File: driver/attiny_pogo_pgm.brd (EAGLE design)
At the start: 26.9 x 17.3 mm, 9 parts, among them IC1 ATTiny85, J1 AVR_SPI_PRG_6NS, P5V TPTP10R

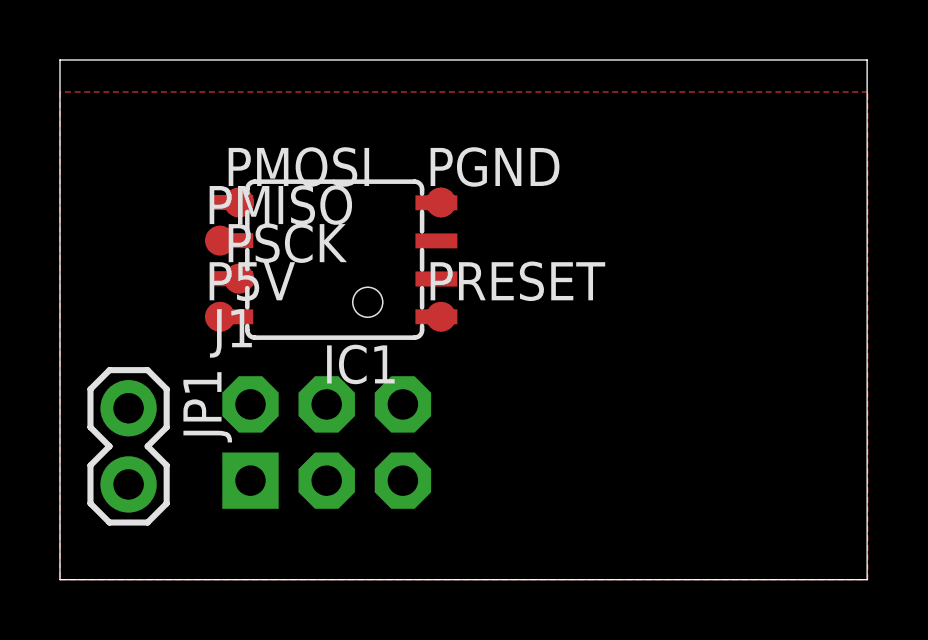
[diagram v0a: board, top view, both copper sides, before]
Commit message: prepare for routing
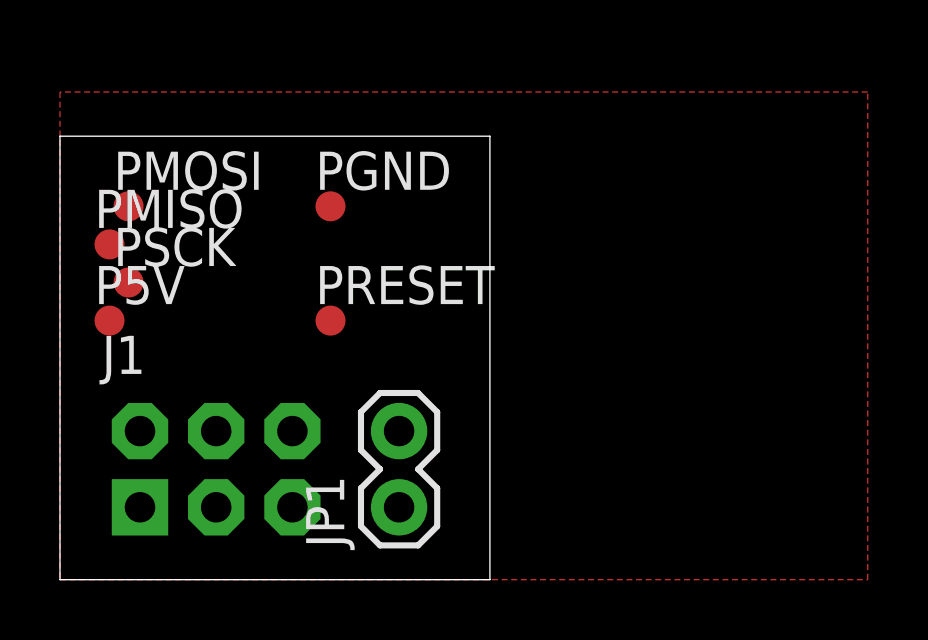
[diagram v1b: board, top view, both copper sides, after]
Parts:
- removed IC1: ATTiny85, atmel:8S2
- moved JP1 9.60 mm to (11.3, 2.41), turned to 90 degrees
- moved J1 3.79 mm to (5.21, 3.68)
- moved PMOSI 3.69 mm to (2.29, 12.4)
- moved PSCK 3.69 mm to (2.29, 9.91)
- moved P5V 3.69 mm to (1.65, 8.64)
- moved PGND 3.69 mm to (9.02, 12.4)
- moved PMISO 3.69 mm to (1.65, 11.2)
- moved PRESET 3.69 mm to (9.02, 8.64)
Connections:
- net +5V: no longer IC1.8
- net GND: no longer IC1.4
- net IN1/MISO: no longer IC1.6
- net RESET-: no longer IC1.1
- net SCL/SCK: no longer IC1.7
- net SDA/MOSI: no longer IC1.5
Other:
- board size 26.9 x 17.3 mm -> 14.3 x 14.8 mm
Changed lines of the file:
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@@
 <board>
 <plain>
-<wire x1="0" y1="0" x2="26.904" y2="0" width="0" layer="20"/>
-<wire x1="26.904" y1="0" x2="26.904" y2="17.323" width="0" layer="20"/>
-<wire x1="26.904" y1="17.323" x2="0" y2="17.323" width="0" layer="20"/>
-<wire x1="0" y1="17.323" x2="0" y2="0" width="0" layer="20"/>
+<wire x1="0" y1="0" x2="14.331" y2="0" width="0" layer="20"/>
+<wire x1="14.331" y1="0" x2="14.331" y2="14.783" width="0" layer="20"/>
+<wire x1="14.331" y1="14.783" x2="0" y2="14.783" width="0" layer="20"/>
+<wire x1="0" y1="14.783" x2="0" y2="0" width="0" layer="20"/>
 </plain>
 <attributes>
@@
 </autorouter>
 <elements>
-<element name="IC1" library="atmel" package="8S2" value="ATTiny85" x="9.144" y="10.668" rot="R90">
-<attribute name="OC_NEWARK" value="96K6522" x="14.224" y="37.338" size="1.778" layer="27" rot="R90" display="off"/>
-<attribute name="MPN" value="ATTINY13-20SU" x="14.224" y="37.338" size="1.778" layer="27" rot="R90" display="off"/>
-<attribute name="MF" value="" x="14.224" y="37.338" size="1.778" layer="27" rot="R90" display="off"/>
-<attribute name="OC_FARNELL" value="9171568" x="14.224" y="37.338" size="1.778" layer="27" rot="R90" display="off"/>
-</element>
-<element name="J1" library="SparkFun-Connectors" package="2X3-NS" value="AVR_SPI_PRG_6NS" x="8.89" y="4.572"/>
-<element name="JP1" library="SparkFun-Connectors" package="1X02" value="" x="2.286" y="5.715" rot="R270"/>
-<element name="PMOSI" library="testpad" package="TP10R" value="TPTP10R" x="5.969" y="12.573">
-<attribute name="TP_SIGNAL_NAME" value="" x="5.969" y="12.573" size="1.778" layer="27" display="off"/>
-</element>
-<element name="PRESET" library="testpad" package="TP10R" value="TPTP10R" x="12.7" y="8.763">
-<attribute name="TP_SIGNAL_NAME" value="" x="12.7" y="8.763" size="1.778" layer="27" display="off"/>
-</element>
-<element name="PSCK" library="testpad" package="TP10R" value="TPTP10R" x="5.969" y="10.033">
-<attribute name="TP_SIGNAL_NAME" value="" x="5.969" y="10.033" size="1.778" layer="27" display="off"/>
-</element>
-<element name="PMISO" library="testpad" package="TP10R" value="TPTP10R" x="5.334" y="11.303">
-<attribute name="TP_SIGNAL_NAME" value="" x="5.334" y="11.303" size="1.778" layer="27" display="off"/>
-</element>
-<element name="PGND" library="testpad" package="TP10R" value="TPTP10R" x="12.7" y="12.573">
-<attribute name="TP_SIGNAL_NAME" value="" x="12.7" y="12.573" size="1.778" layer="27" display="off"/>
-</element>
-<element name="P5V" library="testpad" package="TP10R" value="TPTP10R" x="5.334" y="8.763">
-<attribute name="TP_SIGNAL_NAME" value="" x="5.334" y="8.763" size="1.778" layer="27" display="off"/>
+<element name="J1" library="SparkFun-Connectors" package="2X3-NS" value="AVR_SPI_PRG_6NS" x="5.207" y="3.683"/>
+<element name="JP1" library="SparkFun-Connectors" package="1X02" value="" x="11.303" y="2.413" rot="R90"/>
+<element name="PMOSI" library="testpad" package="TP10R" value="TPTP10R" x="2.286" y="12.446">
+<attribute name="TP_SIGNAL_NAME" value="" x="2.286" y="12.446" size="1.778" layer="27" display="off"/>
+</element>
+<element name="PRESET" library="testpad" package="TP10R" value="TPTP10R" x="9.017" y="8.636">
+<attribute name="TP_SIGNAL_NAME" value="" x="9.017" y="8.636" size="1.778" layer="27" display="off"/>
+</element>
+<element name="PSCK" library="testpad" package="TP10R" value="TPTP10R" x="2.286" y="9.906">
+<attribute name="TP_SIGNAL_NAME" value="" x="2.286" y="9.906" size="1.778" layer="27" display="off"/>
+</element>
+<element name="PMISO" library="testpad" package="TP10R" value="TPTP10R" x="1.651" y="11.176">
+<attribute name="TP_SIGNAL_NAME" value="" x="1.651" y="11.176" size="1.778" layer="27" display="off"/>
+</element>
+<element name="PGND" library="testpad" package="TP10R" value="TPTP10R" x="9.017" y="12.446">
+<attribute name="TP_SIGNAL_NAME" value="" x="9.017" y="12.446" size="1.778" layer="27" display="off"/>
+</element>
+<element name="P5V" library="testpad" package="TP10R" value="TPTP10R" x="1.651" y="8.636">
+<attribute name="TP_SIGNAL_NAME" value="" x="1.651" y="8.636" size="1.778" layer="27" display="off"/>
 </element>
 </elements>
 <signals>
 <signal name="IN1/MISO">
-<contactref element="IC1" pad="6"/>
 <contactref element="J1" pad="1"/>
 <contactref element="PMISO" pad="TP"/>
-<wire x1="5.334" y1="11.303" x2="5.74" y2="11.303" width="0" layer="19" extent="1-1"/>
-<wire x1="6.35" y1="3.302" x2="5.74" y2="11.303" width="0" layer="19" extent="1-1"/>
+<wire x1="2.667" y1="2.413" x2="1.651" y2="11.176" width="0" layer="19" extent="1-1"/>
 </signal>
 <signal name="GND">
-<contactref element="IC1" pad="4"/>
 <contactref element="J1" pad="6"/>
 <polygon width="0.2032" layer="1" isolate="0.4064">
@@
 </signal>
 <signal name="+5V">
-<contactref element="IC1" pad="8"/>
 <contactref element="J1" pad="2"/>
 <contactref element="JP1" pad="1"/>
 <contactref element="P5V" pad="TP"/>
-<wire x1="5.334" y1="8.763" x2="5.74" y2="8.763" width="0" layer="19" extent="1-1"/>
-<wire x1="6.35" y1="5.842" x2="5.74" y2="8.763" width="0" layer="19" extent="1-1"/>
-<wire x1="2.286" y1="5.715" x2="6.35" y2="5.842" width="0" layer="19" extent="1-1"/>
+<wire x1="2.667" y1="4.953" x2="11.303" y2="2.413" width="0" layer="19" extent="1-1"/>
+<wire x1="1.651" y1="8.636" x2="2.667" y2="4.953" width="0" layer="19" extent="1-1"/>
 </signal>
 <signal name="SDA/MOSI">
-<contactref element="IC1" pad="5"/>
 <contactref element="J1" pad="4"/>
 <contactref element="PMOSI" pad="TP"/>
-<wire x1="5.969" y1="12.573" x2="5.74" y2="12.573" width="0" layer="19" extent="1-1"/>
-<wire x1="8.89" y1="5.842" x2="5.969" y2="12.573" width="0" layer="19" extent="1-1"/>
+<wire x1="5.207" y1="4.953" x2="2.286" y2="12.446" width="0" layer="19" extent="1-1"/>
 </signal>
 <signal name="RESET-">
-<contactref element="IC1" pad="1"/>
 <contactref element="J1" pad="5"/>
 <contactref element="PRESET" pad="TP"/>
-<wire x1="12.548" y1="8.763" x2="12.7" y2="8.763" width="0" layer="19" extent="1-1"/>
-<wire x1="11.43" y1="3.302" x2="12.548" y2="8.763" width="0" layer="19" extent="1-1"/>
+<wire x1="7.747" y1="2.413" x2="9.017" y2="8.636" width="0" layer="19" extent="1-1"/>
 </signal>
 <signal name="SCL/SCK">
-<contactref element="IC1" pad="7"/>
 <contactref element="J1" pad="3"/>
 <contactref element="PSCK" pad="TP"/>
-<wire x1="5.969" y1="10.033" x2="5.74" y2="10.033" width="0" layer="19" extent="1-1"/>
-<wire x1="8.89" y1="3.302" x2="5.969" y2="10.033" width="0" layer="19" extent="1-1"/>
+<wire x1="5.207" y1="2.413" x2="2.286" y2="9.906" width="0" layer="19" extent="1-1"/>
 </signal>
 </signals>
